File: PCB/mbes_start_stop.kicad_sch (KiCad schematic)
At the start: 12 parts, among them Q11 BC337, Q13 BC337, Q17 BC327, Q18 BC327, U4 HK19F-DC12-SHG

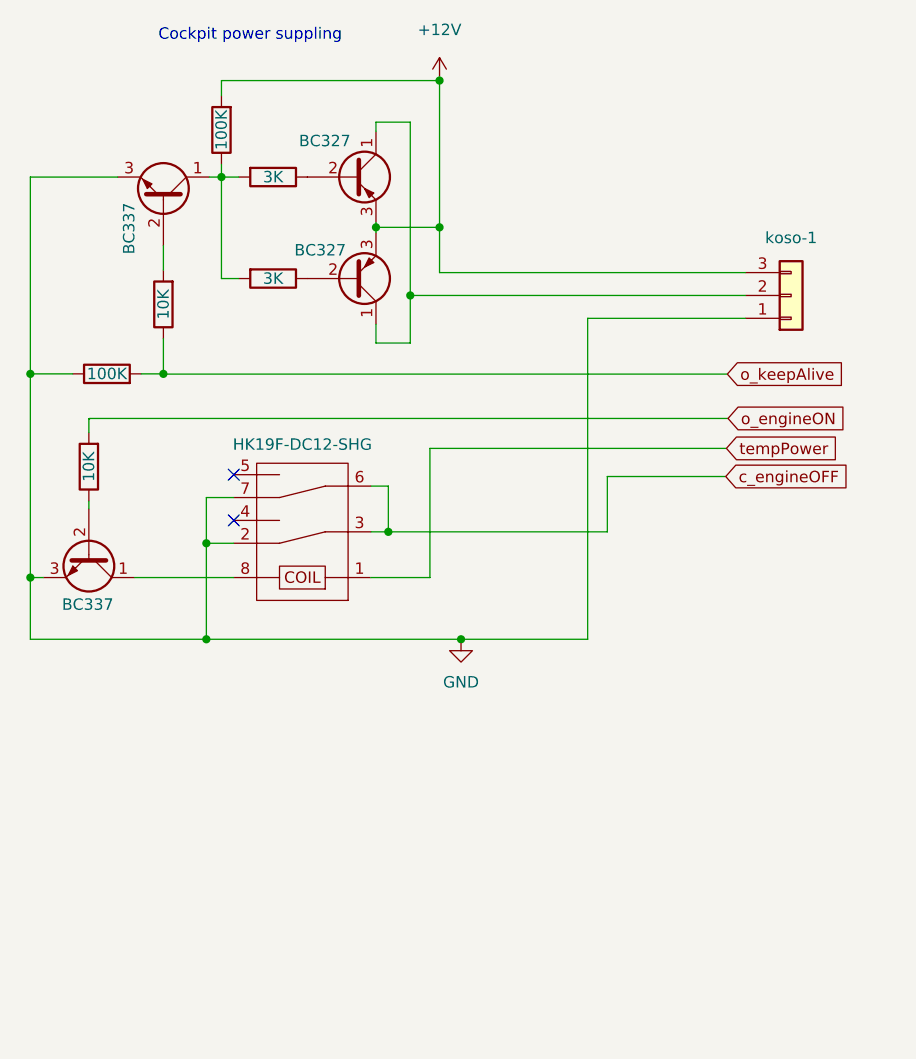
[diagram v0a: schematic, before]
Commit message: Merged files
These files have been merged by remotes/origin/ATmega16__dualPCB__bluetoothCockpit branch
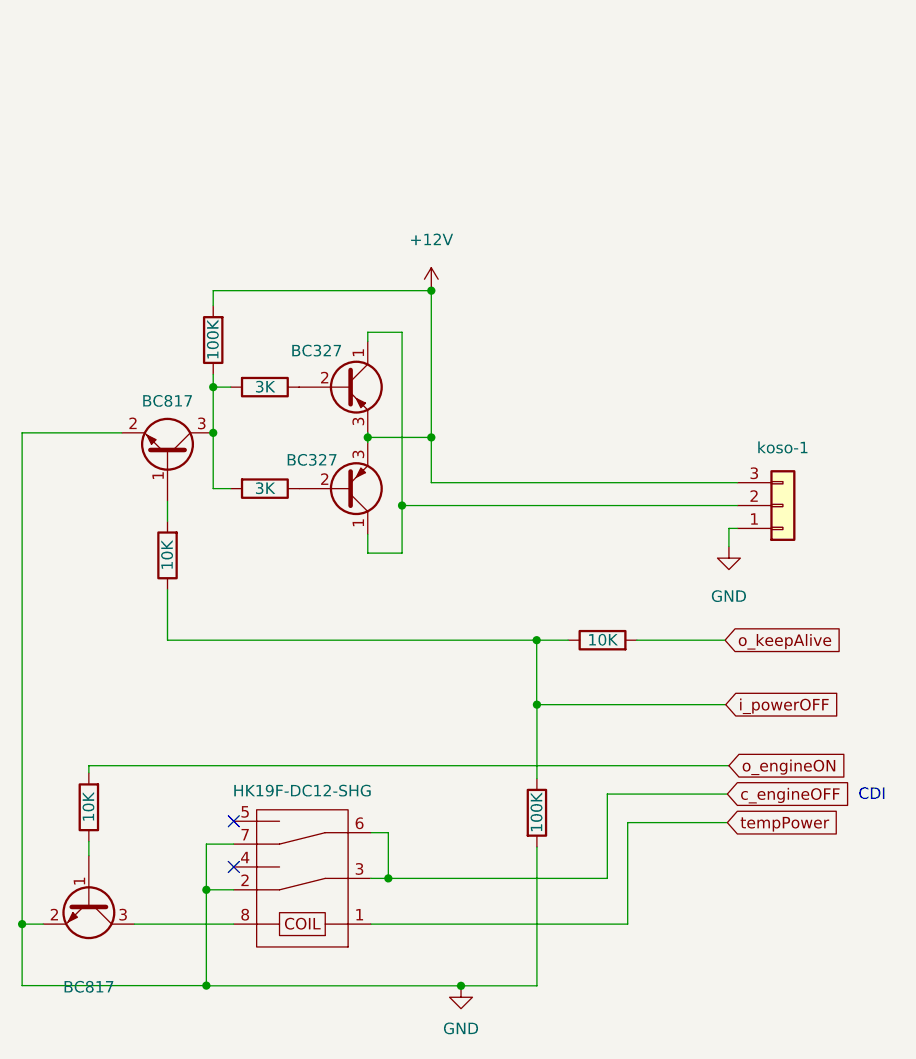
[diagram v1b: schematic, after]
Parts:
- removed Q11, Q13: BC337, Package_TO_SOT_THT:TO-92L_Inline_Wide, symbol Transistor_BJT:BC337
- added Q10, Q12: BC817, Package_TO_SOT_SMD:SOT-23, symbol Transistor_BJT:BC817
- added RA43: 10K, Resistor_SMD:R_1206_3216Metric, symbol Device:R
- RA30, RA31, RA33, RA41, RA44, RA8: footprint Resistor_THT:R_Axial_DIN0207_L6.3mm_D2.5mm_P7.62mm_Horizontal -> Resistor_SMD:R_1206_3216Metric
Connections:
- net GND: now also RA41.2, Q10.2 (E), Q12.2 (E); no longer RA41.1
- net o_keepAlive: now also RA43.2; no longer RA41.2, RA8.1
- net at U4.8: now also Q12.3 (C)
- net at RA44.1: now also Q12.1 (B)
- net at RA30.1, RA31.2, RA33.2: now also Q10.3 (C)
- net at RA8.2: now also Q10.1 (B)
- new net i_powerOFF: RA41.1, RA43.1, RA8.1
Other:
- note added: "CDI"
- note removed: "Cockpit power suppling"
- moved on the sheet: koso-1
